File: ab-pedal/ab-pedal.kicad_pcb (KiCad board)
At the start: 2 copper layers, 96 x 52 mm, 23 parts, among them J1 PEDAL, J2 IN, J4 SEND, J6 RECV, J7 OUT, J8 Jack-DC, SW1 TRUE_BYPASS, SW2 INVERT, SW3 ON, U1 TL074, U2 MAX1044

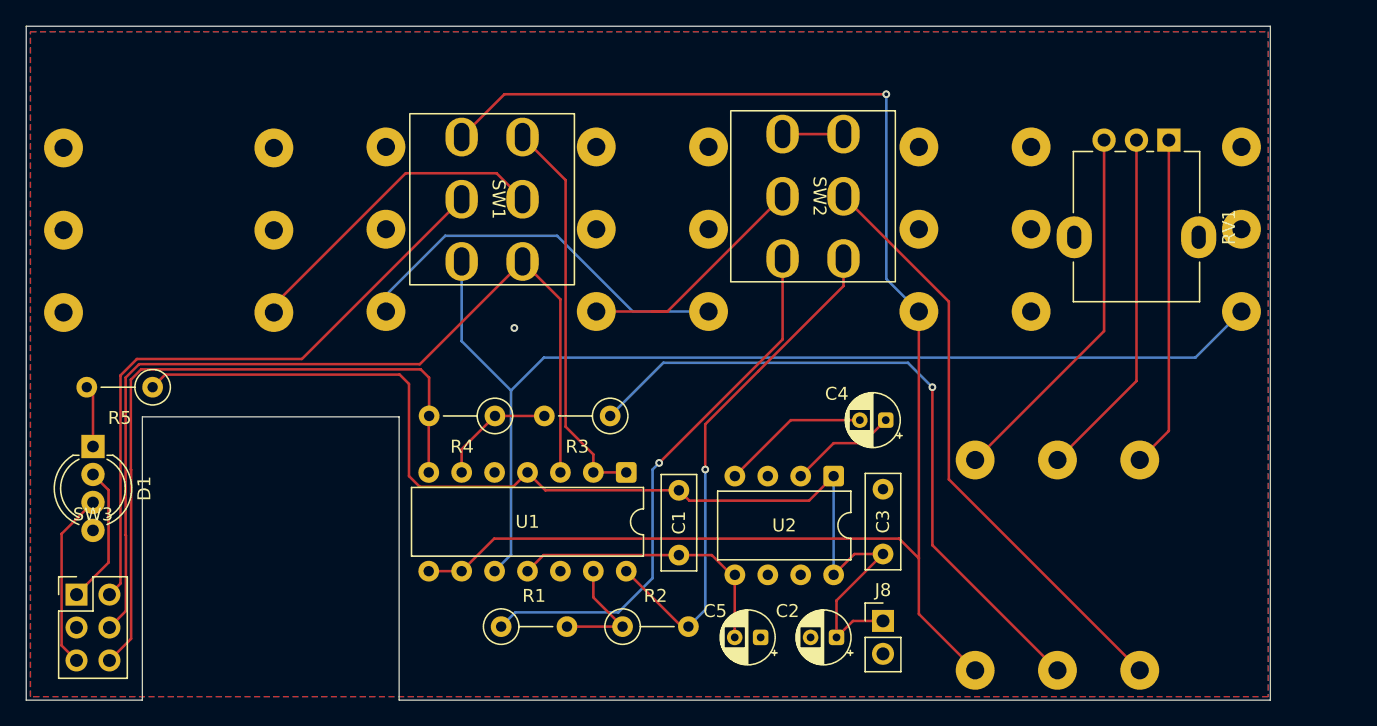
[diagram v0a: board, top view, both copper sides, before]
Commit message: update for mechanicals
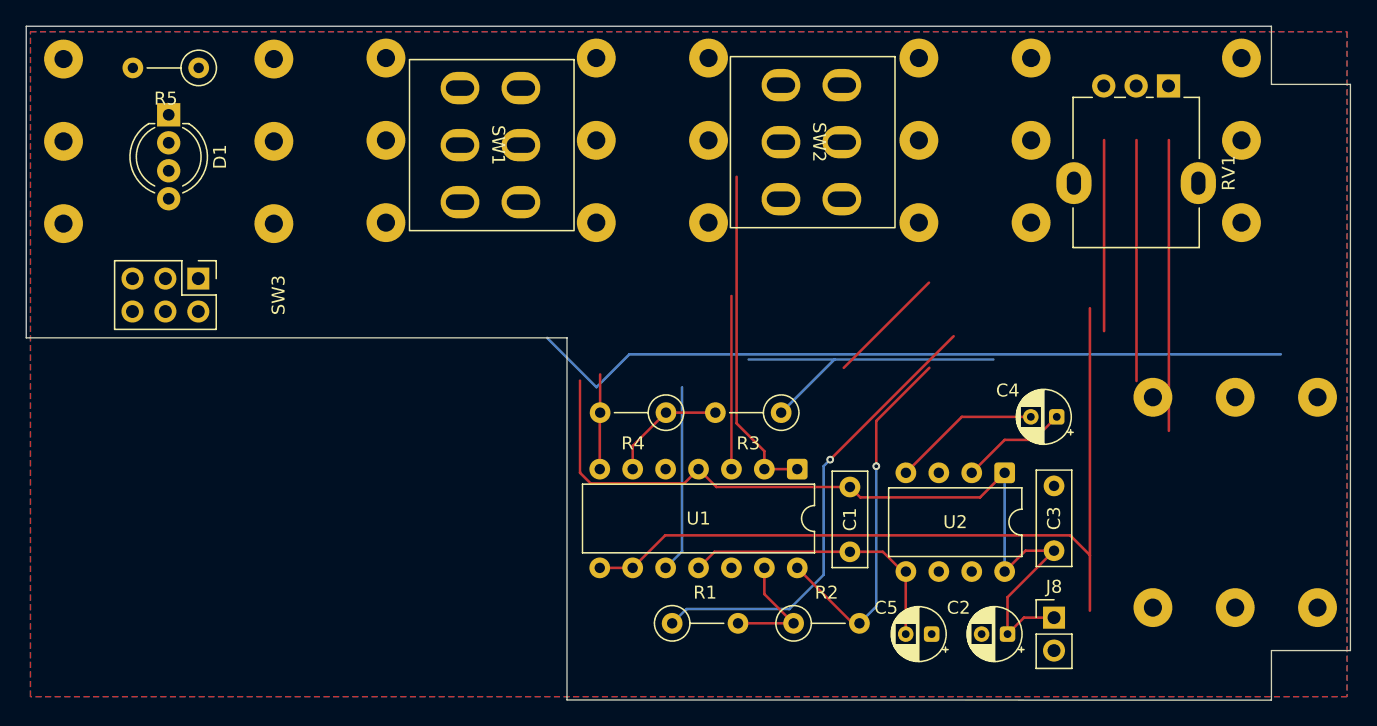
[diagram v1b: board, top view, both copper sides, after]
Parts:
- J1, J2, J4, J6, J7: footprint Connector_Audio:Jack_6.35mm_Neutrik_NMJ6HFD2_Horizontal -> _project:Jack_6.35mm_Neutrik_NMJ6HCD3_Horizontal
- R5: value 1k -> 10k
- moved D1 26.3 mm to (63.0, 80.8)
- moved SW3 26.1 mm to (65.3, 93.5), turned to -90 degrees
- moved R5 24.9 mm to (65.3, 77.2)
- moved J1 14.5 mm to (138.9, 118.9)
- moved C1 13.2 mm to (115.6, 109.6)
- moved C3 13.2 mm to (131.3, 114.5)
- moved C4 13.2 mm to (131.5, 104.1)
- moved C5 13.2 mm to (121.9, 120.9)
- moved J8 13.2 mm to (131.3, 119.6)
- moved U2 13.2 mm to (127.5, 108.5)
- moved R1 13.2 mm to (101.8, 120.1)
- moved R2 13.2 mm to (111.2, 120.1)
- moved R3 13.2 mm to (110.3, 103.8)
- moved R4 13.2 mm to (101.4, 103.8)
- moved U1 13.2 mm to (111.5, 108.2)
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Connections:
- D1 pad 1: Net-(D1-A) -> Net-(D1-BK)
- D1 pad 2: Net-(D1-RK) -> unconnected-(D1-GK-Pad2)
- D1 pad 3: Net-(D1-GK) -> Net-(D1-A)
- D1 pad 4: unconnected-(D1-BK-Pad4) -> Net-(D1-RK)
- SW3 pad 3: Net-(D1-GK) -> Net-(D1-BK)
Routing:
- net Net-(SW1A-C): track 71.6 -> 13.4 mm
- net BUFFERED: track 120.9 -> 62.8 mm, vias 1 -> 0
- net Net-(SW1B-B): track 49.2 -> 0.00 mm
- net RETURN~: track 46.0 -> 0.00 mm
- net BLEND: track 53.3 -> 7.28 mm
- net Net-(J4-PadTN): track 30.5 -> 0.00 mm
- net Net-(J1-PadR): track 53.2 -> 24.7 mm, vias 1 -> 0
- net Net-(J1-PadSN): track 25.6 -> 0.00 mm
- net OUT: track 24.2 -> 0.00 mm
- net +9V: track 87.0 -> 66.5 mm
- net RETURN: track 19.2 -> 0.00 mm
- net Net-(D1-GK): track 13.7 -> 0.00 mm
- net IN: track 84.9 -> 73.7 mm
- net Net-(D1-RK): track 10.8 -> 0.00 mm
- net Net-(J1-PadRN): track 27.2 -> 18.6 mm
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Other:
- board size 96 x 52 mm -> 102.2 x 52 mm
